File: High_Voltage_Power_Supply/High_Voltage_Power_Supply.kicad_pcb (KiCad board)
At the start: 2 copper layers, 220 x 125 mm, 107 parts, among them J1 Conn_01x02_Female, J2 Conn_01x02_Female, J3 Conn_01x02_Female, J4 Conn_01x12_Female, Q1 Q_NMOS_GDS, Q2 Q_NMOS_GDS, Q3 Q_NIGBT_GCE, U1 LT3751-TSSOP, U10 ADR3412, U11 LM2576HVT-15, U2 LT3751-TSSOP, U4 ZXGD3004E6, U5 MC14504B, U6 MC14504B, U7 LM7805, U8 LM7805, U9 LMV331

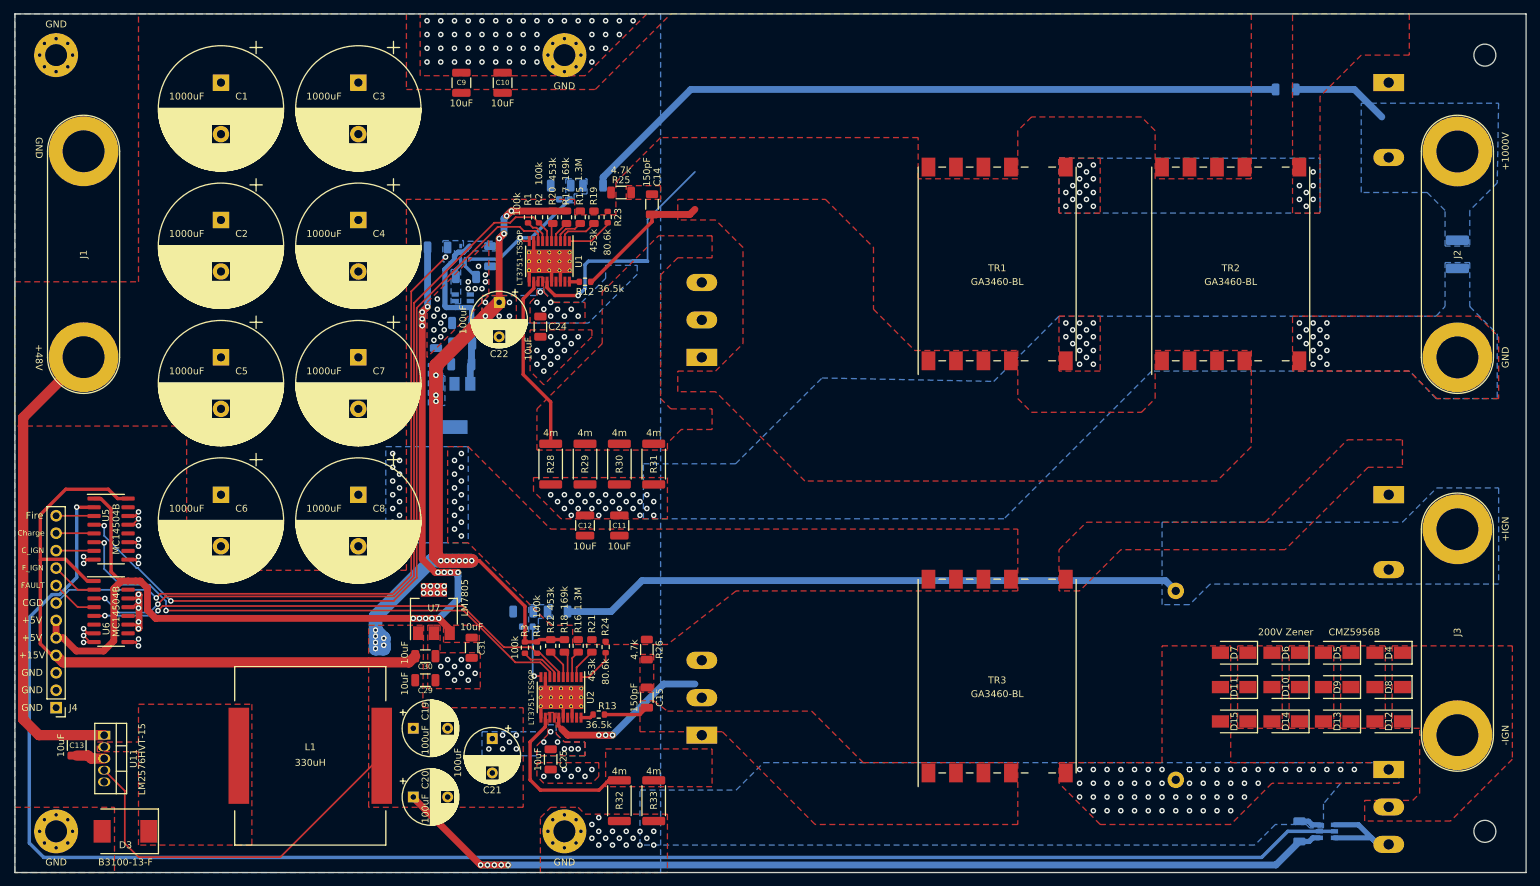
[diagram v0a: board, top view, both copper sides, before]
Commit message: Component updates for new version
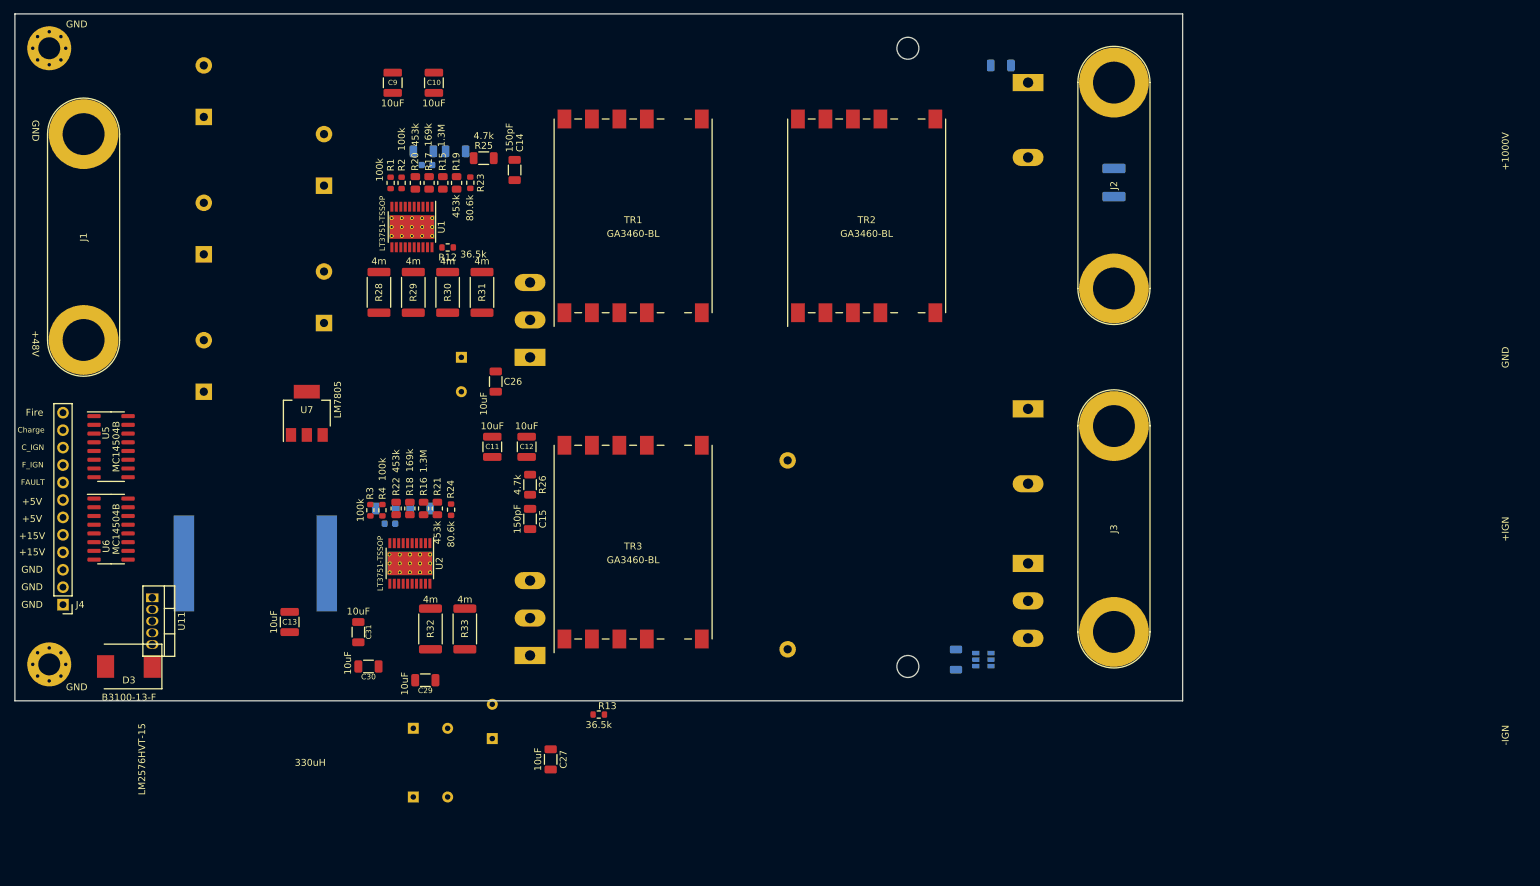
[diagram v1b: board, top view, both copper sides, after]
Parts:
- removed C16, C17: 0.1uF, Capacitor_SMD:C_1206_3216Metric
- removed the C26 at (85.1, 88.0)
- removed the C27 at (89.2, 75.3)
- removed C32, C33: 10uF, Capacitor_SMD:C_1206_3216Metric
- removed C6, C7, C8: 1000uF, Capacitor_THT:CP_Radial_D18.0mm_P7.50mm
- removed D10, D11, D12, D13, D14, D15, D4, D5, D6, D7, D8, D9: CMZ5956B, Diode_SMD:D_SMA
- removed the H4 at (100.0, 159.0)
- removed H5: MountingHole_Pad, MountingHole:MountingHole_3.2mm_M3
- removed R27: 4.7k, Resistor_SMD:R_1206_3216Metric
- removed U10: ADR3412, Package_TO_SOT_SMD:SOT-23-6
- removed U8: LM7805, Package_TO_SOT_SMD:SOT-223-3_TabPin2
- removed U9: LMV331, Package_TO_SOT_SMD:SOT-353_SC-70-5
- C1, C19, C2, C20, C21, C22, C3, C4, C5, L1: moved to B.Cu
- H3: footprint MountingHole:MountingHole_3.2mm_M3_Pad_Via -> MountingHole:MountingHole_3.2mm_M3
- moved H4 87.4 mm to (150.0, 135.0)
- moved Q3 60.5 mm to (167.5, 120.0)
- moved C18 59.6 mm to (132.5, 105.0)
- moved TR3 56.5 mm to (110.0, 117.5)
- moved C28 55.9 mm to (157.0, 134.0)
- moved U4 55.9 mm to (161.0, 134.0)
- moved D2 54.0 mm to (167.5, 97.5)
- moved TR1 53.5 mm to (110.0, 70.0)
- moved TR2 53.5 mm to (144.0, 70.0)
- moved D1 52.5 mm to (167.5, 50.0)
- moved J3 52.2 mm to (180.0, 130.0)
- moved C34 51.1 mm to (180.0, 64.5)
- moved J2 51.0 mm to (180.0, 80.0)
- moved H3 50.0 mm to (150.0, 45.0)
- moved R6 41.6 mm to (163.5, 47.5)
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- renumbered C24 to C26, C25 to C27, H6 to H4
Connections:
- H3 pad 1: GND -> (no net)
- J4 pad 5: +5VD -> VCC
- J4 pad 7: Charged -> +5VD
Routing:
- net VCC: track 415.1 -> 0.00 mm, vias 50 -> 0
- net FIRE: track 247.4 -> 0.00 mm, vias 1 -> 0
- net +5VD: track 159.2 -> 0.00 mm, vias 13 -> 0
- net CHARGE: track 117.1 -> 0.00 mm, vias 2 -> 0
- net ~FAULT~: track 116.3 -> 0.00 mm, vias 2 -> 0
- net Net-(R6-Pad2): track 104.4 -> 0.00 mm
- net Charged: track 102.7 -> 0.00 mm, vias 2 -> 0
- net Net-(C18-Pad1): track 91.0 -> 0.00 mm
- net CHARGE_IGN: track 78.0 -> 0.00 mm, vias 2 -> 0
- net ~FAULT_IGN~: track 73.0 -> 0.00 mm, vias 2 -> 0
- net GND: track 71.0 -> 0.00 mm, vias 254 -> 0
- net Vtrans: track 69.1 -> 0.00 mm, vias 26 -> 0
- net Net-(Q1-Pad1): track 38.2 -> 0.00 mm, vias 1 -> 0
- net Net-(Q2-Pad1): track 26.7 -> 0.00 mm, vias 3 -> 0
- net Net-(Q1-Pad3): track 25.9 -> 0.00 mm
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- removed copper zone on B.Cu, net +5VA
- removed copper zone on F.Cu, net +5VD
- removed copper zone on F.Cu, net /Transformer/in-
- removed copper zone on B.Cu, net /Transformer/out+
- removed copper zone on F.Cu, net /Transformer/out+
- removed copper zone on B.Cu, net Charged
- removed copper zone on B.Cu, net GND
- removed copper zone on F.Cu, net GND
- removed copper zone on F.Cu, net Net-(C14-Pad1)
- removed copper zone on F.Cu, net Net-(C15-Pad1)
- removed copper zone on F.Cu, net Net-(C15-Pad2)
- removed copper zone on B.Cu, net Net-(C17-Pad1)
- removed copper zone on B.Cu, net Net-(C18-Pad1)
- removed copper zone on B.Cu, net Net-(C34-Pad1)
- removed copper zone on B.Cu, net Net-(C35-Pad1)
- removed copper zone on B.Cu, net Net-(C36-Pad1)
- removed copper zone on F.Cu, net Net-(D10-Pad1)
- removed copper zone on F.Cu, net Net-(D10-Pad2)
- removed copper zone on F.Cu, net Net-(D12-Pad2)
- removed copper zone on F.Cu, net Net-(D2-Pad2)
- removed copper zone on F.Cu, net Net-(D3-Pad1)
- removed copper zone on F.Cu, net Net-(J3-Pad1)
- removed copper zone on F.Cu, net Net-(Q1-Pad3)
- removed copper zone on F.Cu, net Net-(Q2-Pad3)
- removed copper zone on B.Cu, net VCC
- removed copper zone on F.Cu, net VCC
- removed copper zone on B.Cu, net Vtrans
- removed copper zone on F.Cu, net Vtrans
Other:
- board size 220 x 125 mm -> 170 x 100 mm
- board text removed: "CGD"
